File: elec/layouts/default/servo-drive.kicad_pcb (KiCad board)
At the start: 4 copper layers, 37.5 x 39.9 mm, 105 parts, among them U2 8Mhz

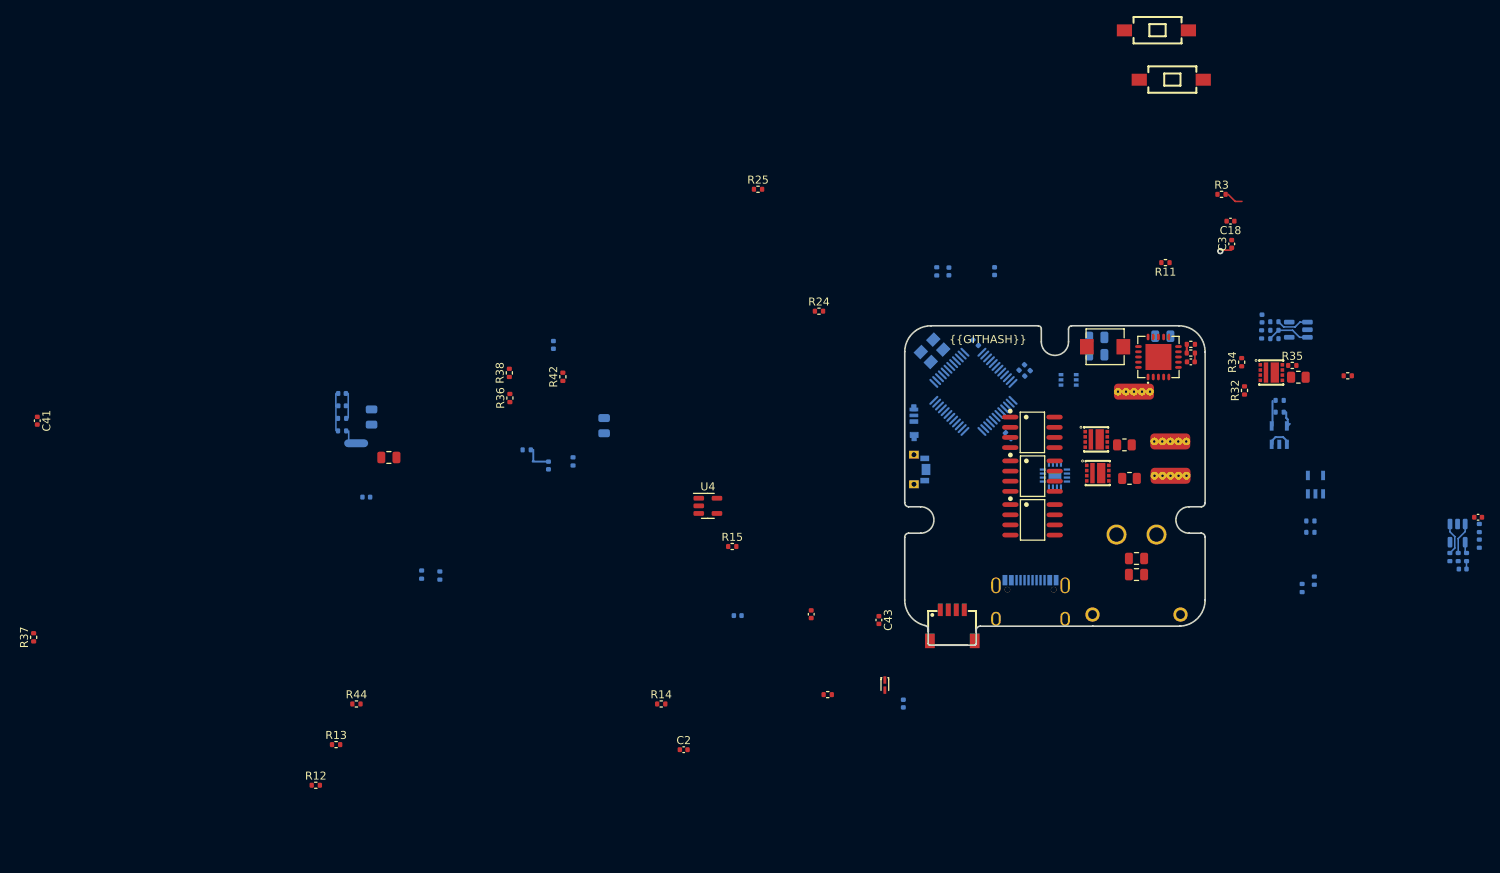
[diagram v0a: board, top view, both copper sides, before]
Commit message: sync layout with ato src
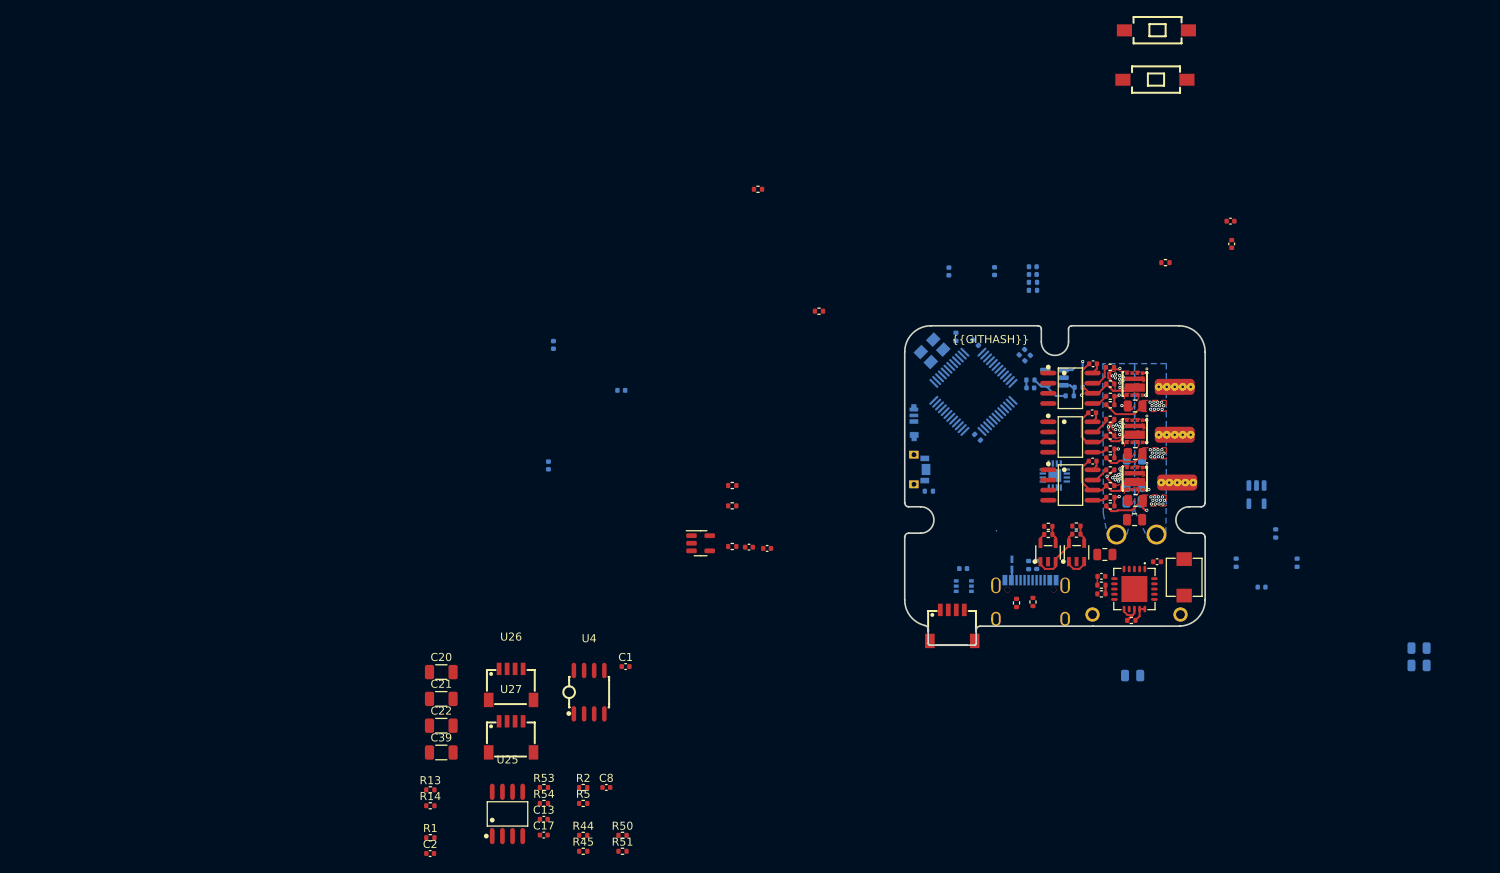
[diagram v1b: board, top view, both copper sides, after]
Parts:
- removed the U17 at (210.9, 119.1)
- added C1: 1uF, Capacitor_SMD:C_0402_1005Metric, F.Cu at (170.1, 124.2)
- added C13: 100nF, Capacitor_SMD:C_0402_1005Metric, F.Cu at (159.8, 143.3)
- added C17: 10nF, Capacitor_SMD:C_0402_1005Metric, F.Cu at (159.8, 145.3)
- added C2: 1uF, Capacitor_SMD:C_0402_1005Metric, F.Cu at (145.6, 147.6)
- added C20: 10uF, Capacitor_SMD:C_1206_3216Metric, F.Cu at (147.0, 124.9)
- added C21: 10uF, Capacitor_SMD:C_1206_3216Metric, F.Cu at (147.0, 128.3)
- added C22: 10uF, Capacitor_SMD:C_1206_3216Metric, F.Cu at (147.0, 131.6)
- added C39: 10uF, Capacitor_SMD:C_1206_3216Metric, F.Cu at (147.0, 135.0)
- added C8: , Capacitor_SMD:C_0402_1005Metric, F.Cu at (167.7, 139.3)
- added R1: 10kOhm, Resistor_SMD:R_0402_1005Metric, F.Cu at (145.7, 145.6)
- added R13: , Resistor_SMD:R_0402_1005Metric, F.Cu at (145.7, 139.6)
- added R2: 10kOhm, Resistor_SMD:R_0402_1005Metric, F.Cu at (164.8, 139.3)
- added R44: , Resistor_SMD:R_0402_1005Metric, F.Cu at (164.8, 145.3)
- added R50: , Resistor_SMD:R_0402_1005Metric, F.Cu at (169.7, 145.3)
- added R51: , Resistor_SMD:R_0402_1005Metric, F.Cu at (169.7, 147.3)
- added R53: 60R, Resistor_SMD:R_0402_1005Metric, F.Cu at (159.8, 139.3)
- added R54: 60R, Resistor_SMD:R_0402_1005Metric, F.Cu at (159.8, 141.3)
- added U25: , lib:SOIC-8_L4.9-W3.9-P1.27-LS6.0-BL, F.Cu at (155.3, 142.7)
- added U26: , lib:CONN-SMD_4P-P1.00_SM04B-SRSS-TB-LF-SN, F.Cu at (155.7, 126.5)
- added U27: , lib:CONN-SMD_4P-P1.00_SM04B-SRSS-TB-LF-SN, F.Cu at (155.7, 133.0)
- added U4: , lib:SOIC-8_L5.0-W4.0-P1.27-LS6.0-BL, F.Cu at (165.5, 127.4)
- C28, D1, R3: moved to B.Cu
- C5, R17, R18, R19, R20, R21, R22, R39, R40, R41, R43, U22, U23: moved to F.Cu
- R14: value 1kOhm -> (none)
- R45: value 1kOhm -> (none); moved to F.Cu
- R49: renamed from R44; moved to B.Cu
- R5: value 1kOhm -> 10kOhm; moved to F.Cu
- moved R37 136.6 mm to (230.6, 97.0), turned to 0 degrees
- moved C41 132.2 mm to (228.5, 86.4), turned to 180 degrees
- moved R49 116.9 mm to (251.3, 107.6), turned to -90 degrees
- moved R45 114.4 mm to (164.8, 147.3), turned to 0 degrees
- moved R5 105.3 mm to (164.8, 141.3)
- moved C44 95.5 mm to (233.7, 98.3), turned to 0 degrees
- moved C40 93.5 mm to (233.7, 105.9)
- moved R27 88.1 mm to (221.0, 77.2)
- moved R28 88.0 mm to (221.0, 76.2)
- moved C33 87.9 mm to (221.0, 75.2)
- moved C34 87.8 mm to (221.0, 74.3)
- moved R19 76.5 mm to (221.0, 116.2)
- moved R38 75.5 mm to (230.6, 95.4), turned to 180 degrees
- moved R36 75.1 mm to (230.6, 93.3), turned to 0 degrees
- moved R39 73.0 mm to (230.6, 98.1), turned to 180 degrees
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- renumbered C1 to C10, C2 to C11, C8 to C12, R2 to R12, R23 to R15, R6 to R16, R24 to R23, R25 to R24, R12 to R25, R13 to R26, R15 to R46, R16 to R47, R26 to R48, R46 to R52, R1 to R6, U24 to U1, U3 to U20, U4 to U21, U20 to U24, U21 to U28, U1 to U3
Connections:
- R14 pad 1: servo_drive.ato:ServoDrive.power_stage.current_sense_b.i_in-half_bridge_b.pwr_gnd -> servo_drive.ato:ServoDrive.power_stage.current_sense_a.bias_div.output-opamp.in_p
- R14 pad 2: servo_drive.ato:ServoDrive.power_stage.current_sense_b.opamp.in_p -> servo_drive.ato:ServoDrive.v_3
- R45 pad 1: servo_drive.ato:ServoDrive.power_stage.current_sense_c.i_in-half_bridge_c.pwr_gnd -> servo_drive.ato:ServoDrive.power_stage.current_sense_b.bias_div.output-opamp.in_p
- R45 pad 2: servo_drive.ato:ServoDrive.power_stage.current_sense_c.opamp.in_p -> servo_drive.ato:ServoDrive.v_3
- R5 pad 1: servo_drive.ato:ServoDrive.power_stage.current_sense_a.i_in-half_bridge_a.pwr_gnd -> servo_drive.ato:ServoDrive.power_stage.reference.buffer.in_p_b-half_ref.output
- R5 pad 2: servo_drive.ato:ServoDrive.power_stage.current_sense_a.opamp.in_p -> servo_drive.ato:ServoDrive.gnd
- U15 pad 45: servo_drive.ato:ServoDrive.micro_kit.micro.PB8 -> servo_drive.ato:ServoDrive.canbus.can_rx
- U15 pad 46: servo_drive.ato:ServoDrive.micro_kit.micro.PB9 -> servo_drive.ato:ServoDrive.canbus.can_tx
- U20 pad 1: servo_drive.ato:ServoDrive.power_stage.current_sense_a.opamp.in_p -> servo_drive.ato:ServoDrive.power_stage.current_sense_a.bias_div.output-opamp.in_p
- U21 pad 1: servo_drive.ato:ServoDrive.power_stage.current_sense_b.opamp.in_p -> servo_drive.ato:ServoDrive.power_stage.current_sense_b.bias_div.output-opamp.in_p
- U24 pad 1: servo_drive.ato:ServoDrive.power_stage.current_sense_c.opamp.in_p -> servo_drive.ato:ServoDrive.power_stage.current_sense_c.bias_div.output-opamp.in_p
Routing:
- net servo_drive.ato:ServoDrive.gnd: track 6.12 -> 30.9 mm, vias 0 -> 38
- net servo_drive.ato:ServoDrive.power_stage.out_a: track 0.00 -> 11.2 mm
- net servo_drive.ato:ServoDrive.power_stage.out_c: track 0.00 -> 11.2 mm
- net servo_drive.ato:ServoDrive.power_stage.out_b: track 0.00 -> 11.2 mm
- net servo_drive.ato:ServoDrive.power_stage.current_sense_a.i_in-half_bridge_a.pwr_gnd: track 0.00 -> 9.10 mm, vias 0 -> 2
- net servo_drive.ato:ServoDrive.power_stage.half_bridge_c.fets.gate_top: track 0.00 -> 9.04 mm, vias 0 -> 2
- net servo_drive.ato:ServoDrive.power_stage.half_bridge_b.fets.gate_top: track 0.00 -> 8.84 mm, vias 0 -> 2
- net servo_drive.ato:ServoDrive.power_stage.half_bridge_a.fets.gate_top: track 0.00 -> 7.65 mm, vias 0 -> 2
- net servo_drive.ato:ServoDrive.power_stage.half_bridge_b.fets.gate_bottom: track 0.00 -> 6.64 mm, vias 0 -> 2
- net servo_drive.ato:ServoDrive.power_stage.half_bridge_c.fets.gate_bottom: track 0.00 -> 6.58 mm, vias 0 -> 2
- net servo_drive.ato:ServoDrive.power_stage.half_bridge_a.fets.gate_bottom: track 0.00 -> 5.67 mm, vias 0 -> 2
- net servo_drive.ato:ServoDrive.v_5: track 2.17 -> 7.50 mm
- net servo_drive.ato:ServoDrive.power_stage.current_sense_a.feedback_div.gnd-opamp.out-output_filter.in: track 0.00 -> 4.72 mm
- net servo_drive.ato:ServoDrive.voltage_input_vdiv.out: track 4.62 -> 0.00 mm
- net servo_drive.ato:ServoDrive.buck.SGND: track 0.92 -> 5.24 mm
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- added copper zone on B.Cu, net servo_drive.ato:ServoDrive.gnd
- added copper zone on F.Cu, net servo_drive.ato:ServoDrive.gnd
- added copper zone on In2.Cu, net servo_drive.ato:ServoDrive.gnd
- added copper zone on F.Cu, net servo_drive.ato:ServoDrive.power_stage.current_sense_a.i_in-half_bridge_a.pwr_gnd
- added copper zone on F.Cu, net servo_drive.ato:ServoDrive.power_stage.current_sense_b.i_in-half_bridge_b.pwr_gnd
- added copper zone on F.Cu, net servo_drive.ato:ServoDrive.power_stage.current_sense_c.i_in-half_bridge_c.pwr_gnd
- added copper zone on B.Cu, net servo_drive.ato:ServoDrive.vbatt
- added copper zone on F.Cu, net servo_drive.ato:ServoDrive.vbatt
- added copper zone on In2.Cu, net servo_drive.ato:ServoDrive.vbatt
